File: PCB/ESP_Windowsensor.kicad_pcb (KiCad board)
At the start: 2 copper layers, 125.7 x 25.4 mm, 6 parts, among them IC1 ATtiny13A-SSU, IC2 ESP-07, Q1 BSP129, SW1 SW_Reed_SPDT

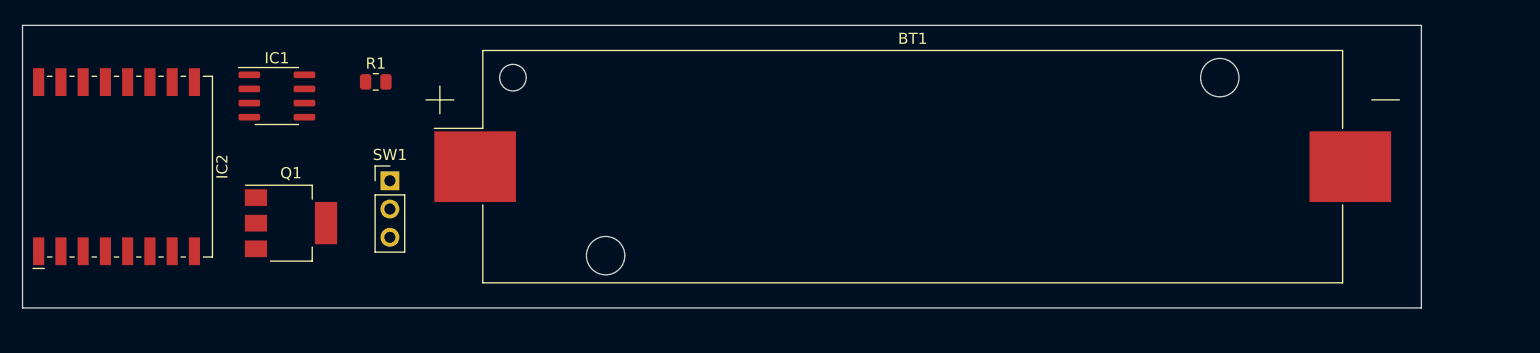
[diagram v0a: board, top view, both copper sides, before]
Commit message: Add files via upload
upload board rev 0.1
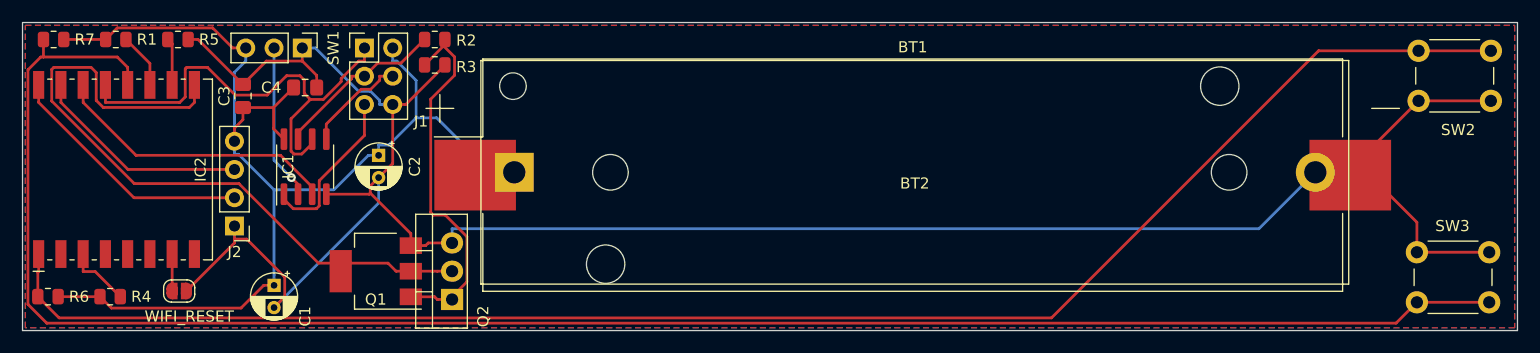
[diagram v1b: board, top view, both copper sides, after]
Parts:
- added BT2: Battery_Cell, Battery:BatteryHolder_MPD_BH-18650-PC2, F.Cu at (93.7, 75.4)
- added C1: 4,7µ, Capacitor_THT:CP_Radial_D4.0mm_P2.00mm, F.Cu at (72.1, 85.6)
- added C2: 4,7µ, Capacitor_THT:CP_Radial_D4.0mm_P2.00mm, F.Cu at (81.5, 73.9)
- added C3: 100n, Capacitor_SMD:C_0805_2012Metric_Pad1.18x1.45mm_HandSolder, F.Cu at (69.3, 68.6)
- added C4: 100n, Capacitor_SMD:C_0805_2012Metric_Pad1.18x1.45mm_HandSolder, F.Cu at (74.9, 67.8)
- added J1: AVR-ISP-6, Connector_PinHeader_2.54mm:PinHeader_2x03_P2.54mm_Vertical, F.Cu at (80.3, 64.3)
- added J2: Conn_01x04_Female, Connector_PinHeader_2.54mm:PinHeader_1x04_P2.54mm_Vertical, F.Cu at (68.6, 80.3)
- added Q2: IRF3708, Package_TO_SOT_THT:TO-220-3_Vertical, F.Cu at (88.1, 86.9)
- added R2: 100, Resistor_SMD:R_0805_2012Metric, F.Cu at (86.6, 63.5)
- added R3: 10k, Resistor_SMD:R_0805_2012Metric, F.Cu at (86.6, 65.8)
- added R4: 10k, Resistor_SMD:R_0805_2012Metric, F.Cu at (57.4, 86.6)
- added R5: 10k, Resistor_SMD:R_0805_2012Metric, F.Cu at (63.5, 63.5)
- added R6: 10k, Resistor_SMD:R_0805_2012Metric, F.Cu at (51.8, 86.6)
- added R7: 10k, Resistor_SMD:R_0805_2012Metric, F.Cu at (52.3, 63.5)
- added SW2: SW_Push, Button_Switch_THT:SW_PUSH_6mm, F.Cu at (175.0, 64.5)
- added SW3: SW_Push, Button_Switch_THT:SW_PUSH_6mm, F.Cu at (181.4, 87.1)
- added WIFI_RESET: SolderJumper_2_Open, Jumper:SolderJumper-2_P1.3mm_Open_RoundedPad1.0x1.5mm, F.Cu at (63.6, 86.1)
- Q1: value BSP129 -> IRLML6244
- moved R1 23.7 mm to (57.9, 63.5)
- moved SW1 14.3 mm to (74.7, 64.3), turned to 270 degrees
- moved Q1 8.76 mm to (81.3, 84.3), turned to 180 degrees
- moved IC1 6.84 mm to (74.9, 74.9), turned to 90 degrees
- moved BT1 0.76 mm to (129.5, 75.7)
- moved IC2 0.25 mm to (55.9, 75.2)
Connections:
- IC1 pad 1: Net-(IC1-Pad1) -> ISP_RST
- IC1 pad 3: ESP_ON -> ESP_READY
- IC1 pad 5: Net-(IC1-Pad5) -> ISP_MOSI
- IC1 pad 6: Net-(IC1-Pad6) -> ISP_MISO
- IC1 pad 7: Net-(IC1-Pad7) -> ISP_SCK
- IC2 pad 1: Net-(IC2-Pad1) -> ESP_RST
- IC2 pad 12: Net-(IC2-Pad12) -> ESP_BOOT
- IC2 pad 13: Net-(IC2-Pad13) -> ISP_MISO
- IC2 pad 14: Net-(IC2-Pad14) -> ESP_READY
- IC2 pad 15: Net-(IC2-Pad15) -> RX
- IC2 pad 16: Net-(IC2-Pad16) -> TX
- IC2 pad 3: +BATT -> Net-(IC2-Pad3)
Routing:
- net GND: track 0.00 -> 206.6 mm
- net ESP_BOOT: track 0.00 -> 166.9 mm
- net ESP_RST: track 0.00 -> 145.2 mm
- net +BATT: track 0.00 -> 111.3 mm
- net Net-(IC2-Pad9): track 0.00 -> 63.5 mm
- net ISP_MISO: track 0.00 -> 41.9 mm
- net ESP_ON: track 0.00 -> 33.6 mm
- net ESP_READY: track 0.00 -> 26.0 mm
- net TX: track 0.00 -> 22.7 mm
- net RX: track 0.00 -> 19.7 mm
- net ISP_SCK: track 0.00 -> 15.6 mm
- net ISP_RST: track 0.00 -> 14.9 mm
- net SENSOR: track 0.00 -> 14.0 mm, vias 0 -> 1
- net ISP_MOSI: track 0.00 -> 9.32 mm
- net Net-(IC2-Pad3): track 0.00 -> 5.85 mm
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- added copper zone on B.Cu, net GND
- added copper zone on F.Cu, net GND
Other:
- board size 125.7 x 25.4 mm -> 134.4 x 27.7 mm
